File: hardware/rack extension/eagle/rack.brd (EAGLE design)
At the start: 160 x 100 mm, 48 parts, among them IC1 74HC139N, IC2 74HC574N, IC3 74HC32N, IC4 74HC86N, IC5 74HC04N, IC6 74HC14N, IC7 74HC541N, K1 APF30212C, K2 APF30212C, Q1 BC547, Q2 BC547, X1 MAC64L

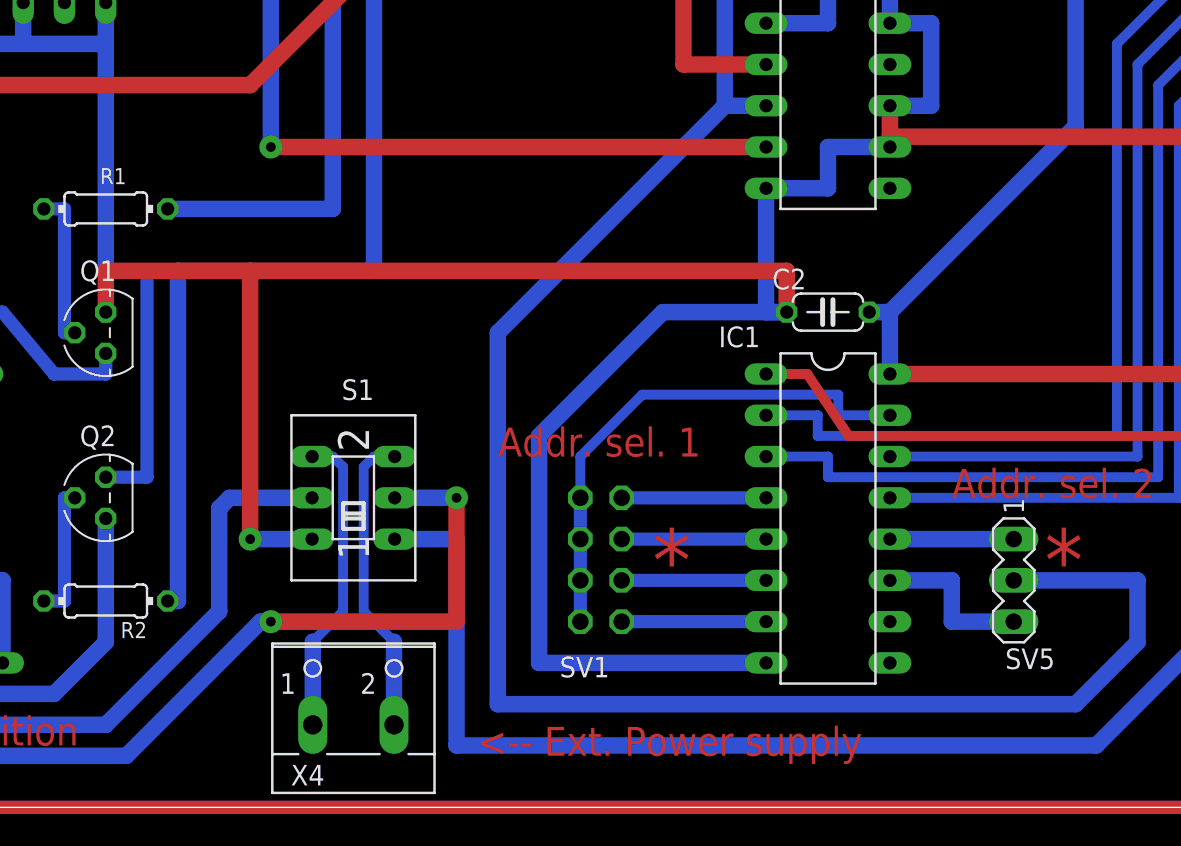
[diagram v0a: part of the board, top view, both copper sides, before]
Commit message: Little layout update
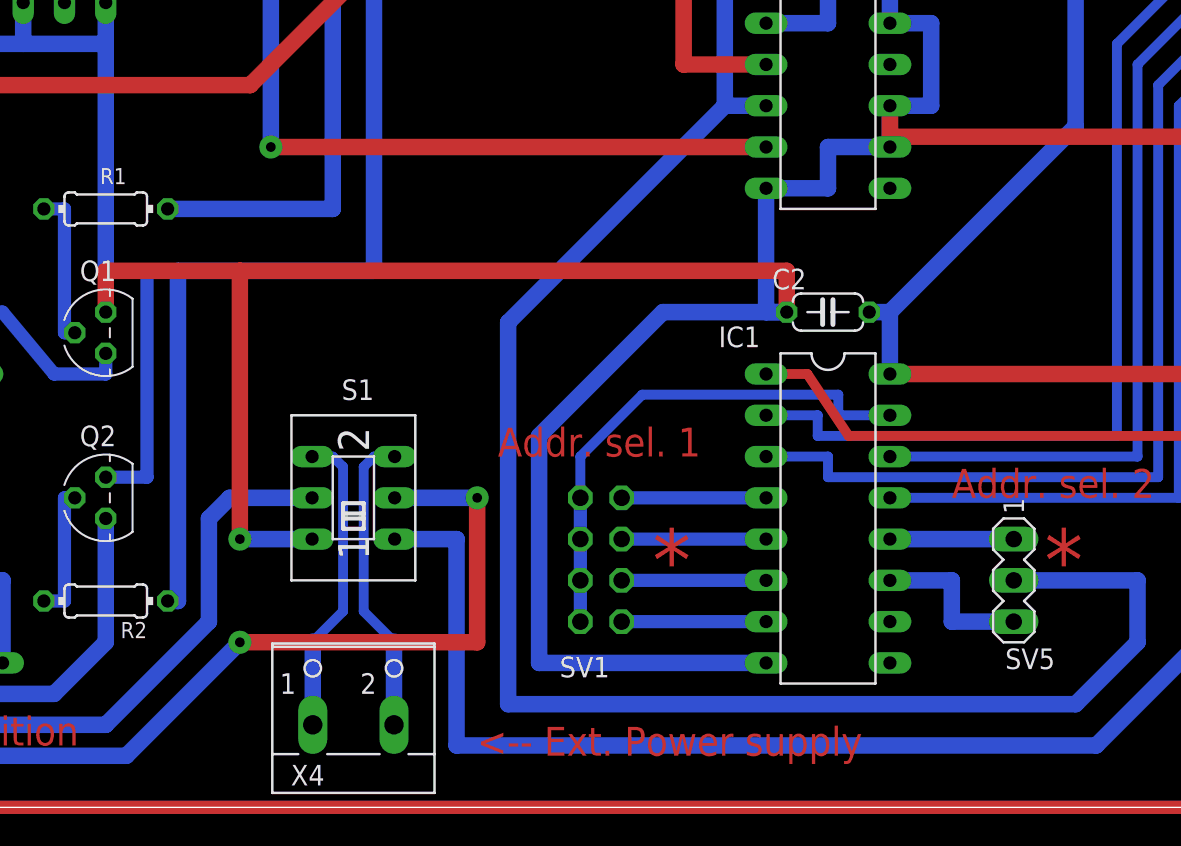
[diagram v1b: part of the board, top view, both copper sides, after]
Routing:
- net N$34: track 78.4 -> 81.7 mm
- net N$36: track 107.7 -> 106.8 mm
- net GND: track 771.6 -> 772.2 mm
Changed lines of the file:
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@@
 <wire x1="118.11" y1="50.8" x2="114.3" y2="50.8" width="1.016" layer="1"/>
 <wire x1="114.3" y1="50.8" x2="114.3" y2="57.15" width="1.016" layer="1"/>
-<wire x1="69.85" y1="33.02" x2="78.74" y2="33.02" width="1.016" layer="1"/>
-<wire x1="78.74" y1="33.02" x2="111.76" y2="33.02" width="1.016" layer="1"/>
+<wire x1="69.85" y1="33.02" x2="78.105" y2="33.02" width="1.016" layer="1"/>
+<wire x1="78.105" y1="33.02" x2="111.76" y2="33.02" width="1.016" layer="1"/>
 <wire x1="111.76" y1="33.02" x2="111.76" y2="30.48" width="1.016" layer="1"/>
 <wire x1="149.86" y1="10.795" x2="154.94" y2="10.795" width="1.016" layer="16"/>
@@
 <wire x1="20.32" y1="66.04" x2="17.78" y2="68.58" width="1.016" layer="16"/>
 <contactref element="S1" pad="4"/>
-<wire x1="82.55" y1="16.51" x2="78.74" y2="16.51" width="1.016" layer="16"/>
-<via x="78.74" y="16.51" extent="1-16" drill="0.6" diameter="1.4224"/>
-<wire x1="78.74" y1="16.51" x2="78.74" y2="33.02" width="1.016" layer="1"/>
+<wire x1="82.55" y1="16.51" x2="78.105" y2="16.51" width="1.016" layer="16"/>
+<via x="78.105" y="16.51" extent="1-16" drill="0.6" diameter="1.4224"/>
+<wire x1="78.105" y1="16.51" x2="78.105" y2="33.02" width="1.016" layer="1"/>
 <wire x1="50.8" y1="66.04" x2="54.61" y2="66.04" width="1.016" layer="1"/>
 <wire x1="54.61" y1="66.04" x2="54.61" y2="85.09" width="1.016" layer="1"/>
@@
 <wire x1="44.47" y1="13.97" x2="44.47" y2="10.16" width="1.016" layer="16"/>
 <wire x1="44.47" y1="10.16" x2="49.55" y2="5.08" width="1.016" layer="16"/>
-<wire x1="69.85" y1="5.08" x2="76.835" y2="12.065" width="1.016" layer="16"/>
-<wire x1="76.835" y1="12.065" x2="76.835" y2="18.415" width="1.016" layer="16"/>
-<wire x1="76.835" y1="18.415" x2="77.47" y2="19.05" width="1.016" layer="16"/>
+<wire x1="69.85" y1="5.08" x2="76.2" y2="11.43" width="1.016" layer="16"/>
+<wire x1="76.2" y1="11.43" x2="76.2" y2="17.78" width="1.016" layer="16"/>
+<wire x1="76.2" y1="17.78" x2="77.47" y2="19.05" width="1.016" layer="16"/>
 <wire x1="77.47" y1="19.05" x2="82.55" y2="19.05" width="1.016" layer="16"/>
 </signal>
@@
 <wire x1="44.45" y1="6.35" x2="47.625" y2="3.175" width="1.016" layer="16"/>
 <wire x1="47.625" y1="3.175" x2="71.12" y2="3.175" width="1.016" layer="16"/>
-<wire x1="87.63" y1="19.05" x2="91.44" y2="19.05" width="1.016" layer="16"/>
-<via x="91.44" y="19.05" extent="1-16" drill="0.6" diameter="1.4224"/>
-<wire x1="91.44" y1="19.05" x2="91.44" y2="11.43" width="1.016" layer="1"/>
-<wire x1="91.44" y1="11.43" x2="80.01" y2="11.43" width="1.016" layer="1"/>
-<via x="80.01" y="11.43" extent="1-16" drill="0.6" diameter="1.4224"/>
-<wire x1="80.01" y1="11.43" x2="79.375" y2="11.43" width="1.016" layer="16"/>
-<wire x1="79.375" y1="11.43" x2="71.12" y2="3.175" width="1.016" layer="16"/>
+<wire x1="87.63" y1="19.05" x2="92.71" y2="19.05" width="1.016" layer="16"/>
+<via x="92.71" y="19.05" extent="1-16" drill="0.6" diameter="1.4224"/>
+<wire x1="92.71" y1="19.05" x2="92.71" y2="10.16" width="1.016" layer="1"/>
+<wire x1="92.71" y1="10.16" x2="78.105" y2="10.16" width="1.016" layer="1"/>
+<via x="78.105" y="10.16" extent="1-16" drill="0.6" diameter="1.4224"/>
+<wire x1="78.105" y1="10.16" x2="71.12" y2="3.175" width="1.016" layer="16"/>
 </signal>
 <signal name="N$30">
@@
 <wire x1="107.95" y1="50.8" x2="110.49" y2="50.8" width="1.016" layer="16"/>
 <wire x1="110.49" y1="43.18" x2="107.95" y2="43.18" width="1.016" layer="16"/>
-<wire x1="93.98" y1="29.21" x2="93.98" y2="6.35" width="1.016" layer="16"/>
-<wire x1="93.98" y1="6.35" x2="129.54" y2="6.35" width="1.016" layer="16"/>
+<wire x1="94.615" y1="29.845" x2="94.615" y2="6.35" width="1.016" layer="16"/>
+<wire x1="94.615" y1="6.35" x2="129.54" y2="6.35" width="1.016" layer="16"/>
 <wire x1="133.35" y1="10.16" x2="133.35" y2="13.97" width="1.016" layer="16"/>
-<wire x1="107.95" y1="43.18" x2="93.98" y2="29.21" width="1.016" layer="16"/>
+<wire x1="107.95" y1="43.18" x2="94.615" y2="29.845" width="1.016" layer="16"/>
 <wire x1="129.54" y1="6.35" x2="133.35" y2="10.16" width="1.016" layer="16"/>
 <contactref element="SV5" pad="2"/>
